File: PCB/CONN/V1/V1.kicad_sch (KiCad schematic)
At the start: 9 parts, among them J1 Conn_01x06_Pin, J2 Conn_01x10_Pin, J3 Conn_ARM_SWD_TagConnect_TC203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, J4 Battery, U1 MCP73831-2-OT

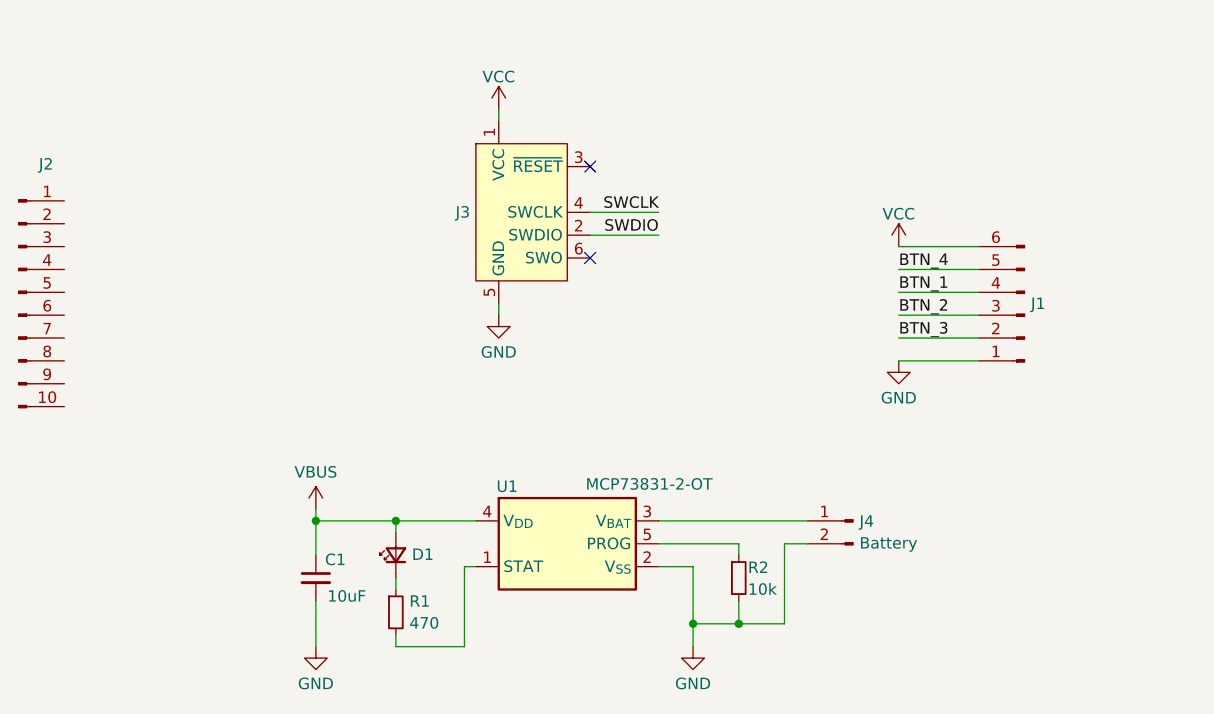
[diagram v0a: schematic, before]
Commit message: udated by FZ
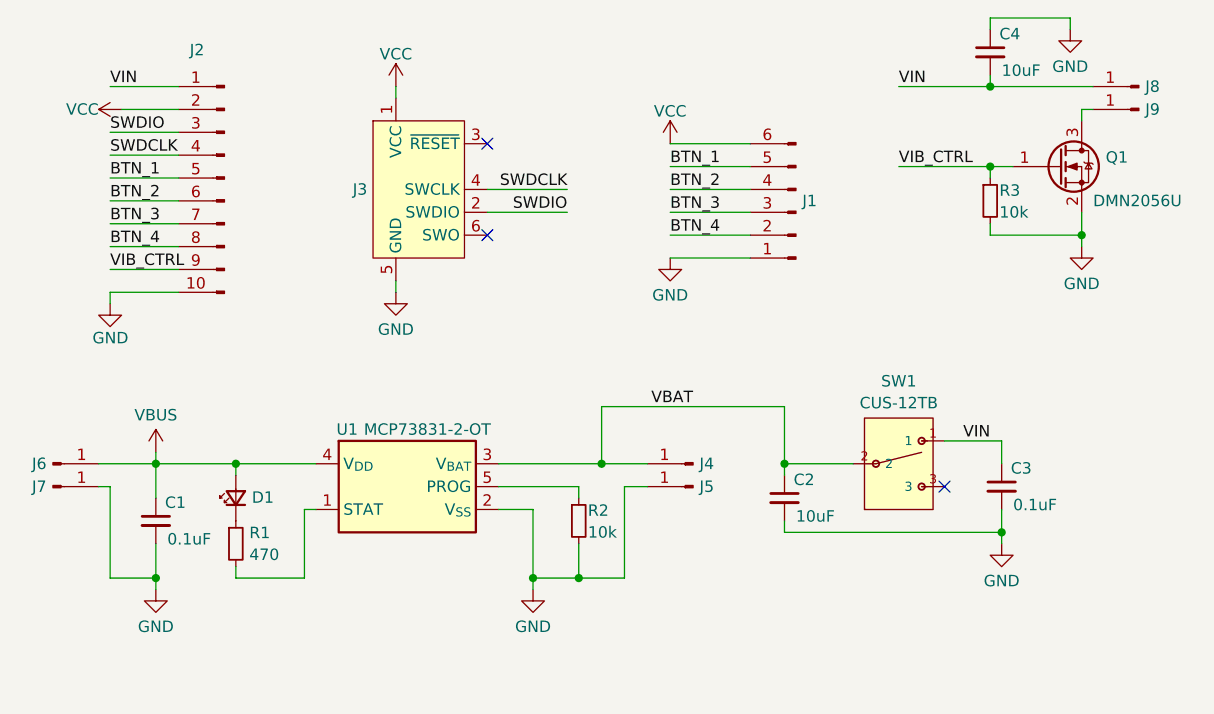
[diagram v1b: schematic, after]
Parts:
- removed J4: Battery, symbol Connector:Conn_01x02_Pin
- added C2, C4: 10uF, Capacitor_SMD:C_0805_2012Metric_Pad1.18x1.45mm_HandSolder, symbol Device:C_Small
- added C3: 0.1uF, Capacitor_SMD:C_0402_1005Metric_Pad0.74x0.62mm_HandSolder, symbol Device:C_Small
- added J4, J5, J6, J7, J8, J9: Conn_01x01_Pin, Mylib:1_pin, symbol Connector:Conn_01x01_Pin
- added Q1: DMN2056U, Package_TO_SOT_SMD:SOT-23, symbol Transistor_FET:DMN2056U
- added R3: 10k, Resistor_SMD:R_0402_1005Metric_Pad0.72x0.64mm_HandSolder, symbol Device:R_Small
- added SW1: CUS-12TB, Mylib:CUS-12B, symbol CUS-12TB:CUS-12TB
- C1: value 10uF -> 0.1uF; footprint (none) -> Capacitor_SMD:C_0402_1005Metric_Pad0.74x0.62mm_HandSolder
- D1: footprint (none) -> LED_SMD:LED_0603_1608Metric_Pad1.05x0.95mm_HandSolder
- J2: footprint (none) -> Mylib:Pinheader_2mmx10
- R1, R2: footprint (none) -> Resistor_SMD:R_0402_1005Metric_Pad0.72x0.64mm_HandSolder
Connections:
- net SWCLK is gone; now on net SWDCLK: J3.4 (SWCLK)
- net BTN_1: now also J1.5 (Pin_5), J2.5 (Pin_5); no longer J1.4 (Pin_4)
- net BTN_2: now also J1.4 (Pin_4), J2.6 (Pin_6); no longer J1.3 (Pin_3)
- net BTN_3: now also J1.3 (Pin_3), J2.7 (Pin_7); no longer J1.2 (Pin_2)
- net BTN_4: now also J1.2 (Pin_2), J2.8 (Pin_8); no longer J1.5 (Pin_5)
- net GND: now also J2.10 (Pin_10), C2.2, C3.2, C4.1, J5.1 (Pin_1), J7.1 (Pin_1), Q1.2 (S), R3.2
- net SWDIO: now also J2.3 (Pin_3)
- net VBUS: now also J6.1 (Pin_1)
- net VCC: now also J2.2 (Pin_2)
- net VBAT: now reaches U1.3 (V_{BAT})
- net VBAT: now also C2.1, J4.1 (Pin_1), SW1.2
- net VIN: now reaches J2.1 (Pin_1)
- net VIN: now also C3.1, C4.2, J8.1 (Pin_1), SW1.1
- net SWDCLK: now reaches J2.4 (Pin_4)
- net VIB_CTRL: now reaches J2.9 (Pin_9)
- net VIB_CTRL: now also Q1.1 (G), R3.1
- new net: J9.1 (Pin_1), Q1.3 (D)
- no-connect marks 2 -> 3
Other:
- moved on the sheet: D1, J1, J2, J3, R1, R2, U1
